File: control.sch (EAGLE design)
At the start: 100 parts, among them CN1 40PIN FPC, CN2 MINI B USB, SW1 TACT, SW10 TACT, SW11 TACT, SW12 TACT, SW13 TACT, SW14 TACT, SW15 TACT, SW16 TACT, SW2 TACT, SW3 TACT, SW4 TACT, SW5 TACT, SW6 TACT, SW7 TACT, SW8 TACT, SW9 TACT, U1 STM32H743ZI, U2 AS4C8M16SA, U3 TPS61169DCKR, U4 USBLC6-2SC6, U5 FT230X, U6 DCDC 3V3

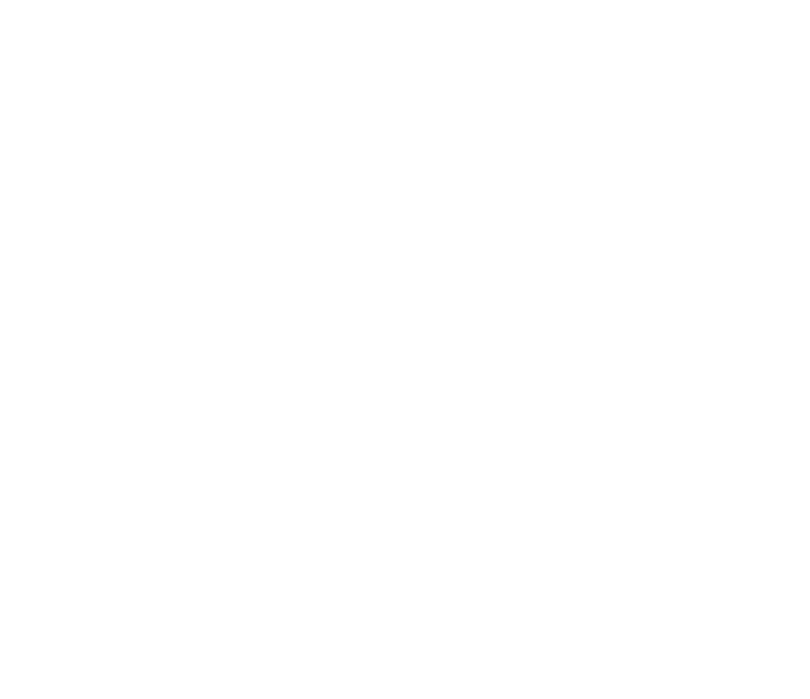
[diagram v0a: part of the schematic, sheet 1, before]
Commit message: Progress
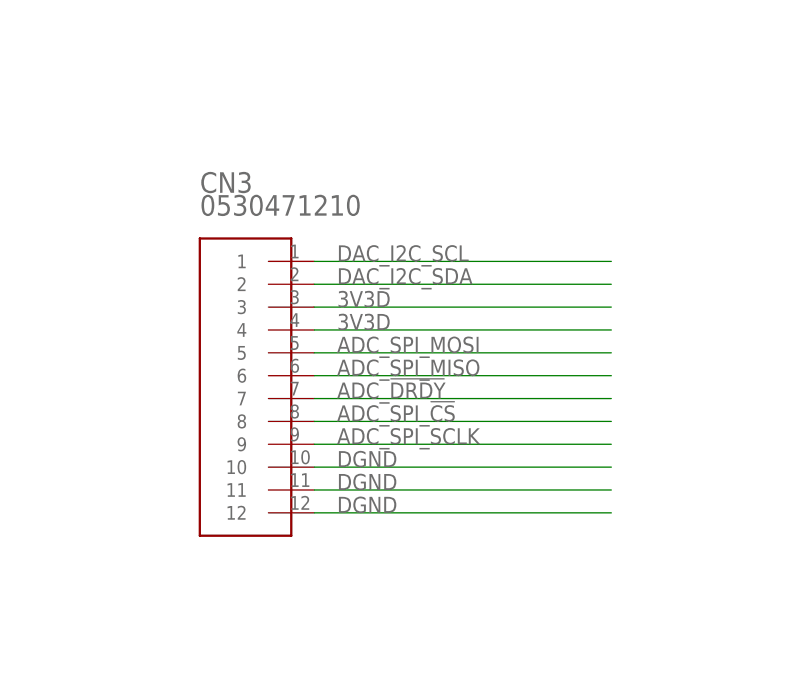
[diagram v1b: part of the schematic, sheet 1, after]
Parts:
- added CN3: 0530471210, CONNECTORs:PICOBLADE_12_TH_V
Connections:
- new net 3V3D: CN3.3, CN3.4
- new net ADC_!DRDY: CN3.7
- new net DGND: CN3.10, CN3.11, CN3.12
- net ADC_SPI_!CS: now also CN3.8
- net ADC_SPI_MISO: now also CN3.6
- net ADC_SPI_MOSI: now also CN3.5
- net ADC_SPI_SCLK: now also CN3.9
- net DAC_I2C_SCL: now also CN3.1
- net DAC_I2C_SDA: now also CN3.2
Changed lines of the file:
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@@
 <part name="GND54" library="NETS" deviceset="GND" device=""/>
 <part name="U$43" library="NETS" deviceset="3V3" device=""/>
+<part name="CN3" library="CONNECTORs" deviceset="PICOBLADE_12_" device="TH_V" value="0530471210"/>
 </parts>
 <sheets>
@@
 <instance part="U$43" gate="G$1" x="-35.56" y="76.2" smashed="yes">
 <attribute name="VALUE" x="-35.56" y="78.74" size="1.778" layer="96" rot="R180" align="center"/>
+</instance>
+<instance part="CN3" gate="G$1" x="231.14" y="325.12" smashed="yes">
+<attribute name="NAME" x="226.06" y="345.44" size="2.286" layer="95"/>
+<attribute name="VALUE" x="226.06" y="342.9" size="2.286" layer="96"/>
 </instance>
 </instances>
@@
 <label x="76.2" y="243.84" size="1.778" layer="95"/>
 </segment>
+<segment>
+<pinref part="CN3" gate="G$1" pin="9"/>
+<wire x1="238.76" y1="317.5" x2="271.78" y2="317.5" width="0.1524" layer="91"/>
+<label x="241.3" y="317.5" size="1.778" layer="95"/>
+</segment>
 </net>
 <net name="ADC_SPI_MOSI" class="0">
@@
 <label x="76.2" y="238.76" size="1.778" layer="95"/>
 </segment>
+<segment>
+<pinref part="CN3" gate="G$1" pin="5"/>
+<wire x1="238.76" y1="327.66" x2="271.78" y2="327.66" width="0.1524" layer="91"/>
+<label x="241.3" y="327.66" size="1.778" layer="95"/>
+</segment>
 </net>
 <net name="N$95" class="0">
@@
 <label x="76.2" y="198.12" size="1.778" layer="95"/>
 </segment>
+<segment>
+<pinref part="CN3" gate="G$1" pin="1"/>
+<wire x1="238.76" y1="337.82" x2="271.78" y2="337.82" width="0.1524" layer="91"/>
+<label x="241.3" y="337.82" size="1.778" layer="95"/>
+</segment>
 </net>
 <net name="DAC_I2C_SDA" class="0">
@@
 <label x="76.2" y="195.58" size="1.778" layer="95"/>
 </segment>
+<segment>
+<pinref part="CN3" gate="G$1" pin="2"/>
+<wire x1="238.76" y1="335.28" x2="271.78" y2="335.28" width="0.1524" layer="91"/>
+<label x="241.3" y="335.28" size="1.778" layer="95"/>
+</segment>
 </net>
 <net name="N$111" class="0">
@@
 <label x="147.32" y="187.96" size="1.778" layer="95"/>
 </segment>
+<segment>
+<pinref part="CN3" gate="G$1" pin="8"/>
+<wire x1="238.76" y1="320.04" x2="271.78" y2="320.04" width="0.1524" layer="91"/>
+<label x="241.3" y="320.04" size="1.778" layer="95"/>
+</segment>
 </net>
 <net name="ADC_SPI_MISO" class="0">
@@
 <wire x1="144.78" y1="190.5" x2="175.26" y2="190.5" width="0.1524" layer="91"/>
 <label x="147.32" y="190.5" size="1.778" layer="95"/>
+</segment>
+<segment>
+<pinref part="CN3" gate="G$1" pin="6"/>
+<wire x1="238.76" y1="325.12" x2="271.78" y2="325.12" width="0.1524" layer="91"/>
+<label x="241.3" y="325.12" size="1.778" layer="95"/>
 </segment>
 </net>
@@
 </segment>
 </net>
+<net name="DGND" class="0">
+<segment>
+<pinref part="CN3" gate="G$1" pin="10"/>
+<wire x1="238.76" y1="314.96" x2="271.78" y2="314.96" width="0.1524" layer="91"/>
+<label x="241.3" y="314.96" size="1.778" layer="95"/>
+</segment>
+<segment>
+<pinref part="CN3" gate="G$1" pin="11"/>
+<wire x1="238.76" y1="312.42" x2="271.78" y2="312.42" width="0.1524" layer="91"/>
+<label x="241.3" y="312.42" size="1.778" layer="95"/>
+</segment>
+<segment>
+<pinref part="CN3" gate="G$1" pin="12"/>
+<wire x1="238.76" y1="309.88" x2="271.78" y2="309.88" width="0.1524" layer="91"/>
+<label x="241.3" y="309.88" size="1.778" layer="95"/>
+</segment>
+</net>
+<net name="3V3D" class="0">
+<segment>
+<pinref part="CN3" gate="G$1" pin="3"/>
+<wire x1="238.76" y1="332.74" x2="271.78" y2="332.74" width="0.1524" layer="91"/>
+<label x="241.3" y="332.74" size="1.778" layer="95"/>
+</segment>
+<segment>
+<pinref part="CN3" gate="G$1" pin="4"/>
+<wire x1="238.76" y1="330.2" x2="271.78" y2="330.2" width="0.1524" layer="91"/>
+<label x="241.3" y="330.2" size="1.778" layer="95"/>
+</segment>
+</net>
+<net name="ADC_!DRDY" class="0">
+<segment>
+<pinref part="CN3" gate="G$1" pin="7"/>
+<wire x1="238.76" y1="322.58" x2="271.78" y2="322.58" width="0.1524" layer="91"/>
+<label x="241.3" y="322.58" size="1.778" layer="95"/>
+</segment>
+</net>
